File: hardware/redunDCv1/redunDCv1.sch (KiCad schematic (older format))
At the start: 16 parts, among them J1 PS1_ALARM, J10 OUT1.4, J11 OUT1.5, J12 OUT1.6, J13 OUT2.1, J14 OUT2.2, J15 OUT2.3, J16 OUT2.4, J2 PS1_PWR, J3 PS1_BAT, J4 PS2_ALARM, J5 PS2_PWR, J6 PS2_BAT, J7 OUT1.1, J8 OUT1.2, J9 OUT1.3

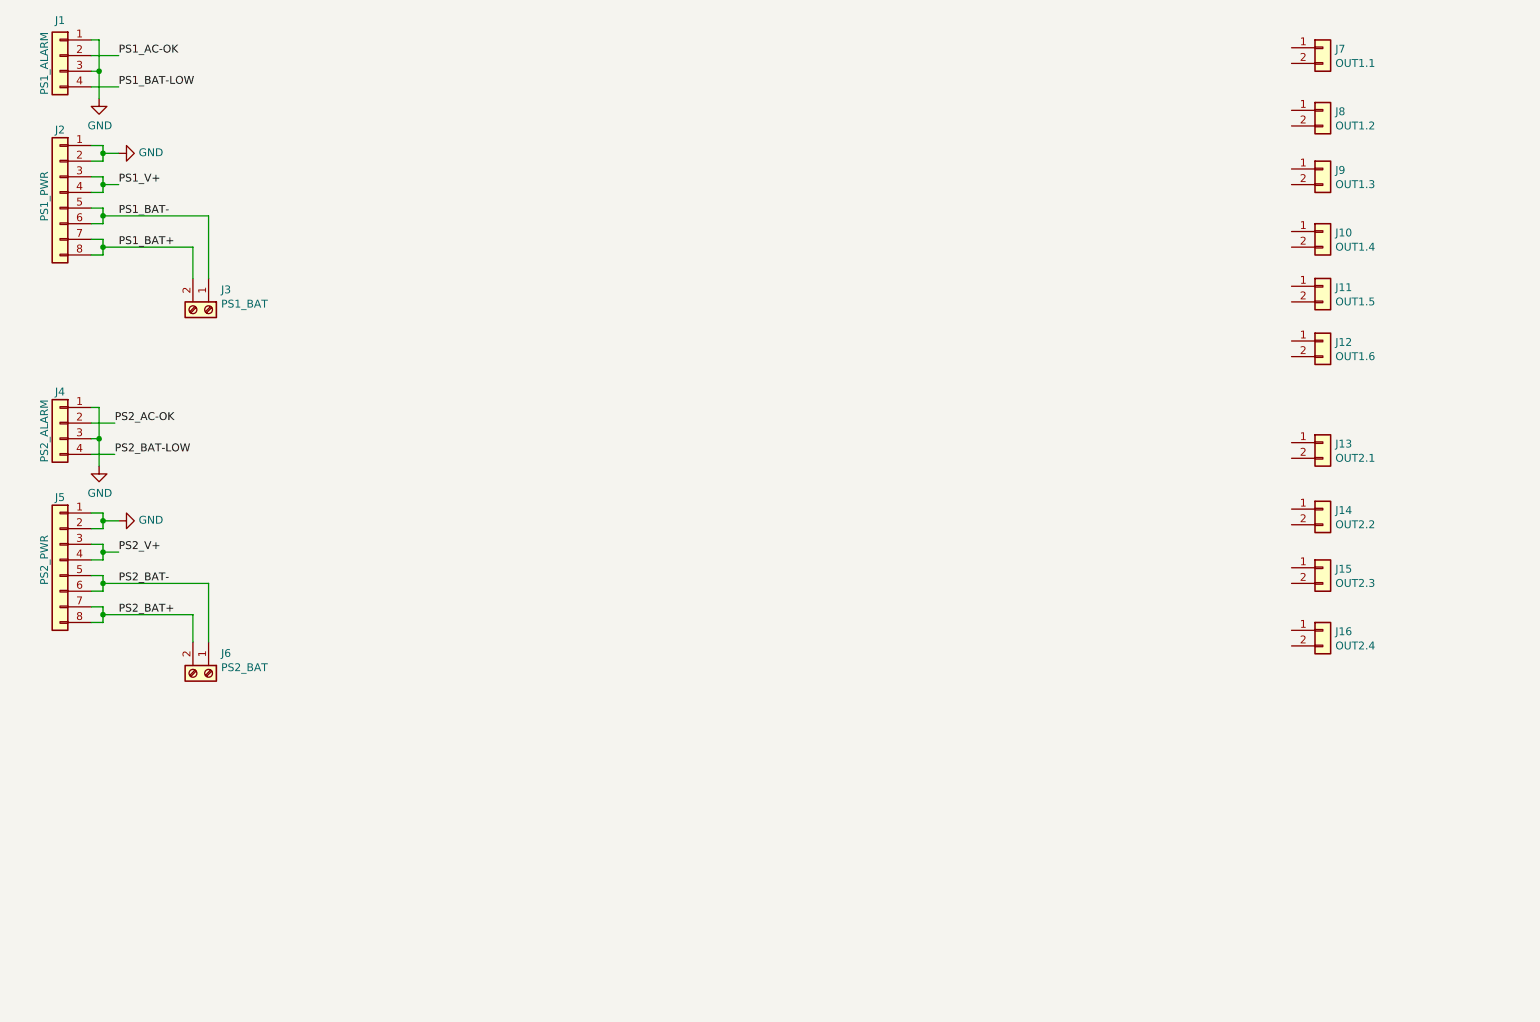
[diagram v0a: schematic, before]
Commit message: first miniamal schematic is done
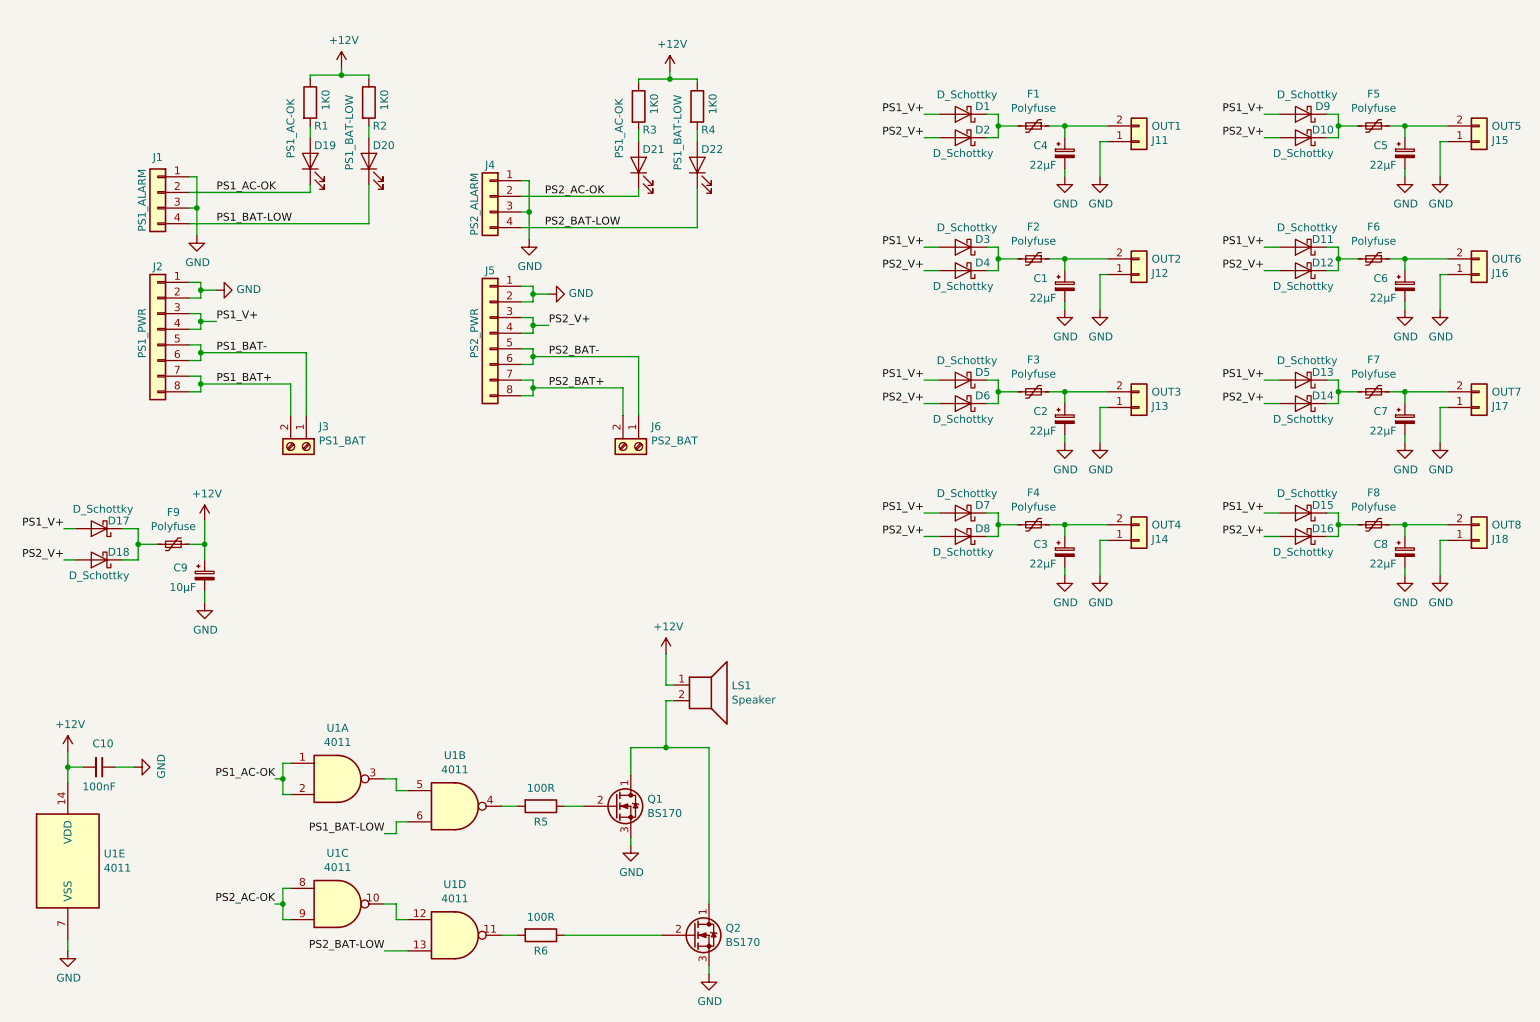
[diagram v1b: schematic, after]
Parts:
- removed J10: OUT1.4, symbol Connector_Generic:Conn_01x02
- removed J11: OUT1.5, symbol Connector_Generic:Conn_01x02
- removed J8: OUT1.2, symbol Connector_Generic:Conn_01x02
- removed J9: OUT1.3, symbol Connector_Generic:Conn_01x02
- added C1, C2, C3, C4, C5, C6, C7, C8: 22µF, symbol Device:CP_Small
- added C10: 100nF, symbol Device:C_Small
- added C9: 10µF, symbol Device:CP_Small
- added D1, D10, D11, D12, D13, D14, D15, D16, D17, D18, D2, D3, D4, D5, D6, D7, D8, D9: D_Schottky, symbol Device:D_Schottky
- added D19, D21: PS1_AC-OK, symbol Device:LED
- added D20, D22: PS1_BAT-LOW, symbol Device:LED
- added F1, F2, F3, F4, F5, F6, F7, F8, F9: Polyfuse, symbol Device:Polyfuse_Small
- added J17: OUT7, symbol Connector_Generic:Conn_01x02
- added J18: OUT8, symbol Connector_Generic:Conn_01x02
- added LS1: Speaker, symbol Device:Speaker
- added Q1, Q2: BS170, Package_TO_SOT_THT:TO-92_Inline, symbol Transistor_FET:BS170
- added R1, R2, R3, R4: 1K0, symbol Device:R
- added R5, R6: 100R, symbol Device:R
- added U1: 4011, symbol 4xxx:4011
- J11: renamed from J7; value OUT1.1 -> OUT1
- J12: value OUT1.6 -> OUT2
- J13: value OUT2.1 -> OUT3
- J14: value OUT2.2 -> OUT4
- J15: value OUT2.3 -> OUT5
- J16: value OUT2.4 -> OUT6
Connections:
- net GND: now also J11.1 (Pin_1), J12.1 (Pin_1), J13.1 (Pin_1), J14.1 (Pin_1), J15.1 (Pin_1), J16.1 (Pin_1), C1.2, C10.1, C2.2, C3.2, C4.2, C5.2, C6.2, C7.2, C8.2, C9.2, J17.1 (Pin_1), J18.1 (Pin_1), Q1.3 (S), Q2.3 (S), U1.7 (VSS)
- net PS1_AC-OK: now also D19.1 (K), U1.1, U1.2
- net PS1_BAT-LOW: now also D20.1 (K), U1.6
- net PS1_V+: now also D1.2 (A), D11.2 (A), D13.2 (A), D15.2 (A), D17.2 (A), D3.2 (A), D5.2 (A), D7.2 (A), D9.2 (A)
- net PS2_AC-OK: now also D21.1 (K), U1.8, U1.9
- net PS2_BAT-LOW: now also D22.1 (K), U1.13
- net PS2_V+: now also D10.2 (A), D12.2 (A), D14.2 (A), D16.2 (A), D18.2 (A), D2.2 (A), D4.2 (A), D6.2 (A), D8.2 (A)
- net at J11.2 (Pin_2): now also C4.1, F1.1
- net at J12.2 (Pin_2): now also C1.1, F2.1
- net at J13.2 (Pin_2): now also C2.1, F3.1
- net at J14.2 (Pin_2): now also C3.1, F4.1
- net at J15.2 (Pin_2): now also C5.1, F5.1
- net at J16.2 (Pin_2): now also C6.1, F6.1
- new net: D1.1 (K), D2.1 (K), F1.2
- new net: D3.1 (K), D4.1 (K), F2.2
- new net: D5.1 (K), D6.1 (K), F3.2
- new net: D7.1 (K), D8.1 (K), F4.2
- new net: D10.1 (K), D9.1 (K), F5.2
- new net: D11.1 (K), D12.1 (K), F6.2
- new net: C7.1, F7.1, J17.2 (Pin_2)
- new net: D13.1 (K), D14.1 (K), F7.2
- new net: C8.1, F8.1, J18.2 (Pin_2)
- new net: D15.1 (K), D16.1 (K), F8.2
- new net: D17.1 (K), D18.1 (K), F9.2
- new net: D19.2 (A), R1.2
- new net: D20.2 (A), R2.2
- new net: D21.2 (A), R3.2
- new net: D22.2 (A), R4.2
- new net: U1.3, U1.5
- new net: R5.2, U1.4
- new net: U1.10, U1.12
- new net: R6.2, U1.11
- new net: LS1.2, Q1.1 (D), Q2.1 (D)
- new net: Q1.2 (G), R5.1
- new net: Q2.2 (G), R6.1
- new net +12V: C10.2, C9.1, F9.1, LS1.1, R1.1, R2.1, R3.1, R4.1, U1.14 (VDD)
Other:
- moved on the sheet: J1, J11, J2, J3, J4, J5, J6
